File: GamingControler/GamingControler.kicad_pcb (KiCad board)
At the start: 2 copper layers, 52 x 55 mm, 48 parts, among them J1 USB_C_Receptacle_USB2.0_16P, J2 USB_C_Receptacle_USB2.0_16P, SW1 SW_Push, SW2 SW_Push, U1 ESP32-C6-WROOM-1, U2 AZ1117-3.3, U3 CP2102N-Axx-xQFN20, U4 TTP223-BA6, U5 TTP223-BA6, U6 TTP223-BA6, U7 TTP223-BA6

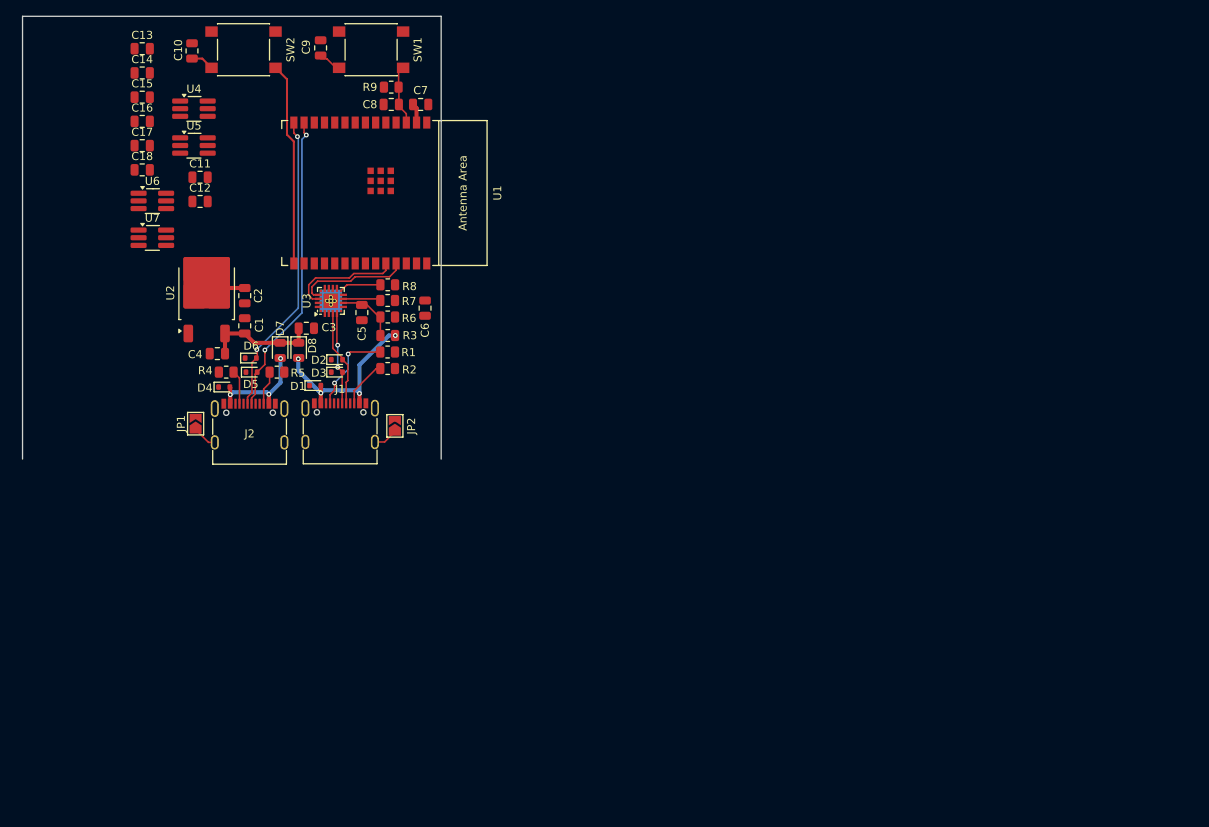
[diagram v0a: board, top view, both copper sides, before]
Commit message: Gaming controller
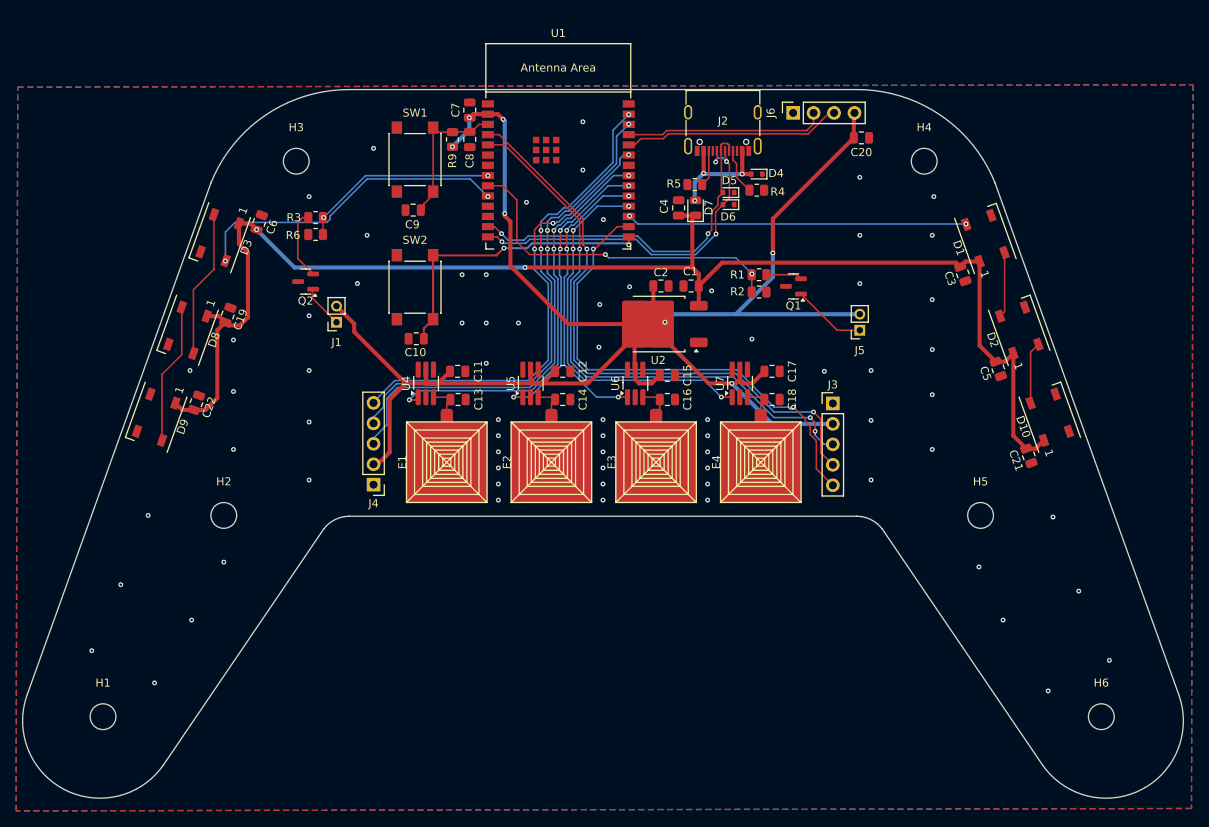
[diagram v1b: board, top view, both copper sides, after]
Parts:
- removed JP1, JP2: SolderJumper_2_Open, Jumper:SolderJumper-2_P1.3mm_Open_TrianglePad1.0x1.5mm
- removed R7: 1K, Resistor_SMD:R_0805_2012Metric
- removed R8: 10K, Resistor_SMD:R_0805_2012Metric
- removed U3: CP2102N-Axx-xQFN20, Package_DFN_QFN:SiliconLabs_QFN-20-1EP_3x3mm_P0.5mm_EP1.8x1.8mm_ThermalVias
- added C19: 100nF, Capacitor_SMD:C_0805_2012Metric, F.Cu at (48.5, 77.1)
- added C20: 100nF, Capacitor_SMD:C_0805_2012Metric, F.Cu at (127.2, 55.1)
- added C21: 100nF, Capacitor_SMD:C_0805_2012Metric, F.Cu at (148.0, 94.6)
- added C22: 100nF, Capacitor_SMD:C_0805_2012Metric, F.Cu at (44.6, 88.0)
- added D10: WS2812B, LED_SMD:LED_WS2812B_PLCC4_5.0x5.0mm_P3.2mm, F.Cu at (150.6, 89.8)
- added D9: WS2812B, LED_SMD:LED_WS2812B_PLCC4_5.0x5.0mm_P3.2mm, F.Cu at (39.6, 89.8)
- added E1: ~, LED_SMD:Electrode_10x10mm, F.Cu at (70.7, 95.4)
- added E2: ~, LED_SMD:Electrode_10x10mm, F.Cu at (83.7, 95.4)
- added E3: ~, LED_SMD:Electrode_10x10mm, F.Cu at (96.7, 95.4)
- added E4: ~, LED_SMD:Electrode_10x10mm, F.Cu at (109.7, 95.4)
- added H1: MountingHole, MountingHole:MountingHole_3.2mm_M3, F.Cu at (33.0, 127.0)
- added H2: MountingHole, MountingHole:MountingHole_3.2mm_M3, F.Cu at (48.0, 102.0)
- added H3: MountingHole, MountingHole:MountingHole_3.2mm_M3, F.Cu at (57.0, 58.0)
- added H4: MountingHole, MountingHole:MountingHole_3.2mm_M3, F.Cu at (135.0, 58.0)
- added H5: MountingHole, MountingHole:MountingHole_3.2mm_M3, F.Cu at (142.0, 102.0)
- added H6: MountingHole, MountingHole:MountingHole_3.2mm_M3, F.Cu at (157.0, 127.0)
- added J3: Conn_01x05_Pin, Connector_PinHeader_2.54mm:PinHeader_1x05_P2.54mm_Vertical, F.Cu at (123.7, 88.1)
- added J4: Conn_01x05_Pin, Connector_PinHeader_2.54mm:PinHeader_1x05_P2.54mm_Vertical, F.Cu at (66.6, 98.2)
- added J5: Conn_01x02_Pin, Connector_PinSocket_2.00mm:PinSocket_1x02_P2.00mm_Vertical, F.Cu at (127.0, 79.0)
- added J6: Conn_01x04_Pin, Connector_PinSocket_2.54mm:PinSocket_1x04_P2.54mm_Vertical, F.Cu at (118.7, 52.0)
- added Q1: NPN, Package_TO_SOT_SMD:SOT-23, F.Cu at (118.8, 73.5)
- added Q2: NPN, Package_TO_SOT_SMD:SOT-23, F.Cu at (58.2, 73.0)
- C3, C5, C6: value 10uF -> 100nF
- D1, D2, D3: value LESD5D5.0CT1G -> WS2812B; footprint Diode_SMD:D_SOD-523 -> LED_SMD:LED_WS2812B_PLCC4_5.0x5.0mm_P3.2mm
- D8: value D -> WS2812B; footprint Diode_SMD:D_0805_2012Metric -> LED_SMD:LED_WS2812B_PLCC4_5.0x5.0mm_P3.2mm
- J1: value USB_C_Receptacle_USB2.0_16P -> Conn_01x02_Pin; footprint Connector_USB:USB_C_Receptacle_G-Switch_GT-USB-7010ASV -> Connector_PinSocket_2.00mm:PinSocket_1x02_P2.00mm_Vertical
- R1, R2: value 5K1 -> R
- R3: value 22.1K -> R
- R6: value 47.5k -> R
- moved D1 85.2 mm to (142.6, 67.6), turned to 109.75 degrees
- moved D2 84.8 mm to (146.8, 79.0), turned to 109.75 degrees
- moved C18 83.3 mm to (116.1, 87.6), turned to 180 degrees
- moved C17 83.1 mm to (116.1, 84.1)
- moved C3 81.8 mm to (139.8, 72.0), turned to 109.75 degrees
- moved C5 79.4 mm to (144.2, 83.8), turned to 109.75 degrees
- moved U7 75.2 mm to (112.1, 85.6), turned to 90 degrees
- moved C15 73.8 mm to (103.1, 84.6)
- moved C16 73.8 mm to (103.1, 87.6), turned to 180 degrees
- moved D4 71.2 mm to (114.2, 59.6), turned to 180 degrees
- moved J2 70.5 mm to (110.0, 53.0), turned to 180 degrees
- moved R4 69.7 mm to (114.2, 61.6), turned to 0 degrees
- moved C14 66.1 mm to (90.1, 87.6), turned to 180 degrees
- moved U6 64.1 mm to (99.1, 85.6), turned to 90 degrees
- moved D5 63.3 mm to (110.7, 61.9), turned to 180 degrees
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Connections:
- C3 pad 1: +5V -> GND
- C3 pad 2: GND -> +5V
- C5 pad 1: Net-(U3-VBUS) -> GND
- C5 pad 2: GND -> +5V
- C6 pad 1: +3V3 -> GND
- C6 pad 2: GND -> +5V
- D1 pad 1: GND -> +5V
- D1 pad 2: VBUSA -> Net-(D1-DOUT)
- D2 pad 1: GND -> +5V
- D2 pad 2: D+ -> Net-(D10-DIN)
- D3 pad 1: GND -> +5V
- D3 pad 2: D- -> Net-(D3-DOUT)
- D8 pad 2: VBUSA -> Net-(D8-DOUT)
- J2 pad S1: Net-(J2-SHIELD) -> GND
- R1 pad 1: Net-(J1-CC1) -> RIGHT_MOTOR
- R1 pad 2: GND -> Net-(Q1-B)
- R2 pad 1: Net-(J1-CC2) -> GND
- R2 pad 2: GND -> RIGHT_MOTOR
- R3 pad 1: VBUSA -> LEFT_MOTOR
- R3 pad 2: Net-(U3-VBUS) -> Net-(Q2-B)
- R6 pad 2: Net-(U3-VBUS) -> LEFT_MOTOR
- U1 pad 10: unconnected-(U1-GPIO8-Pad10) -> LED_DOUT_L
- U1 pad 16: unconnected-(U1-GPIO18-Pad16) -> Push_L
- U1 pad 17: unconnected-(U1-GPIO19-Pad17) -> LED_DOUT_R
- U1 pad 18: unconnected-(U1-GPIO20-Pad18) -> OUTPUT4
- U1 pad 19: unconnected-(U1-GPIO21-Pad19) -> OUTPUT3
- U1 pad 20: unconnected-(U1-GPIO22-Pad20) -> OUTPUT2
- U1 pad 21: unconnected-(U1-GPIO23-Pad21) -> OUTPUT1
- U1 pad 23: OUTPUT -> Push_R
- U1 pad 24: USB_UART_TX -> UART0_RX
- U1 pad 25: USB_UART_RX -> UART0_TX
- U1 pad 26: unconnected-(U1-GPIO3/ADC1_CH3-Pad26) -> V_X_R
- U1 pad 27: unconnected-(U1-GPIO2/ADC1_CH2-Pad27) -> V_Y_R
- U1 pad 4: unconnected-(U1-MTMS/GPIO4/ADC1_CH4-Pad4) -> V_Y_L
- U1 pad 5: unconnected-(U1-MTDI/GPIO5/ADC1_CH5-Pad5) -> V_X_L
- U1 pad 8: unconnected-(U1-GPIO0/ADC1_CH0/XTAL_32K_P-Pad8) -> LEFT_MOTOR
- U1 pad 9: unconnected-(U1-GPIO1/ADC1_CH1/XTAL_32K_N-Pad9) -> RIGHT_MOTOR
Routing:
- net +3V3: track 6.06 -> 215.5 mm, vias 0 -> 7
- net +5V: track 14.0 -> 174.3 mm, vias 0 -> 2
- net V_Y_L: track 0.00 -> 74.6 mm, vias 0 -> 2
- net V_X_L: track 0.00 -> 71.1 mm, vias 0 -> 3
- net V_X_R: track 0.00 -> 64.1 mm, vias 0 -> 3
- net V_Y_R: track 0.00 -> 63.3 mm, vias 0 -> 3
- net Push_L: track 0.00 -> 61.1 mm, vias 0 -> 2
- net Push_R: track 0.00 -> 56.9 mm, vias 0 -> 3
- net OUTPUT1: track 0.00 -> 50.6 mm, vias 0 -> 4
- net OUTPUT4: track 0.00 -> 47.3 mm, vias 0 -> 4
- net RIGHT_MOTOR: track 0.00 -> 42.5 mm, vias 0 -> 2
- net LED_DOUT_R: track 0.00 -> 42.2 mm, vias 0 -> 2
- net LED_DOUT_L: track 0.00 -> 40.1 mm, vias 0 -> 2
- net OUTPUT2: track 0.00 -> 36.6 mm, vias 0 -> 4
- net OUTPUT3: track 0.00 -> 36.1 mm, vias 0 -> 4
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- added copper zone on B.Cu, net GND
- added copper zone on F.Cu, net GND
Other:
- board size 52 x 55 mm -> 144.2 x 88 mm
- board text added: "1"
